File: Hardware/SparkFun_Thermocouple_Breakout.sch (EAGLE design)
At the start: 16 parts, among them U1 MAX31855K

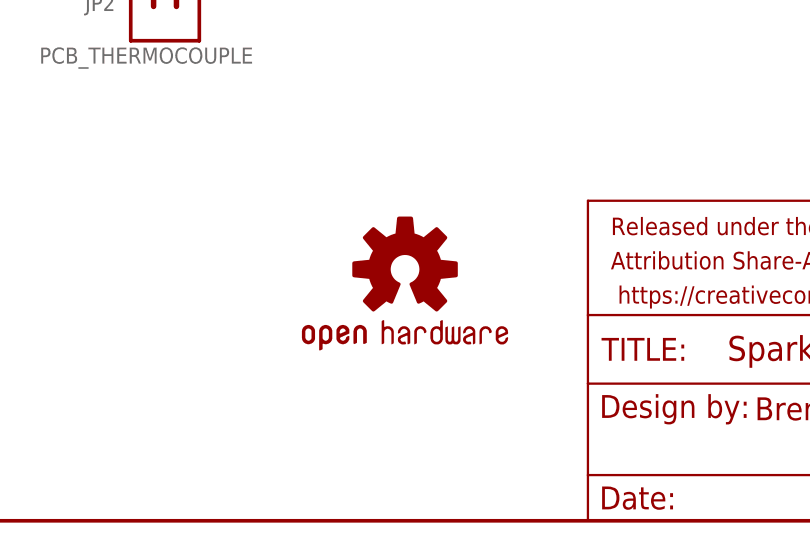
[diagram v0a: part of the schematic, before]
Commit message: Added more logos!
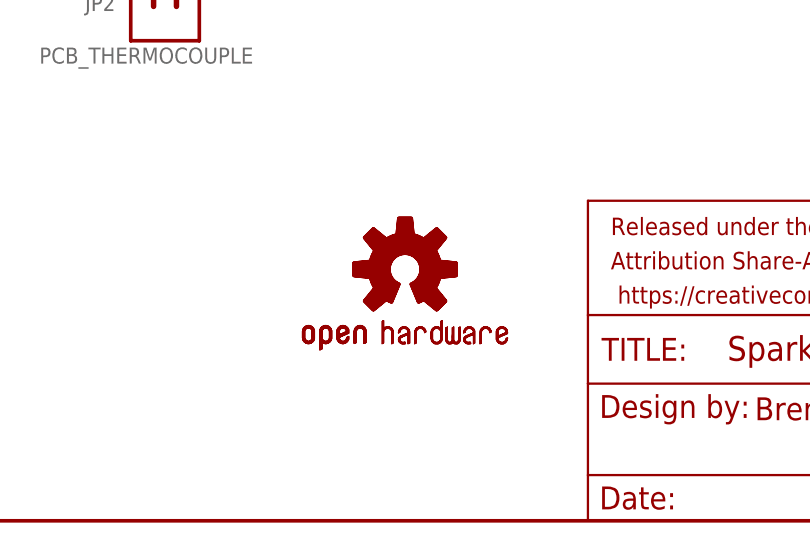
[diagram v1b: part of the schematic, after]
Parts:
- added LOGO4: OSHW-LOGOS, SparkFun-Aesthetics:OSHW-LOGOS
- U1: PROD_ID (none) -> IC-12578
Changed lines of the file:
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@@
 <part name="FID2" library="SparkFun-Aesthetics" deviceset="FIDUCIAL" device="1X2"/>
 <part name="C1" library="SparkFun-Capacitors" deviceset="0.1UF-25V(+80/-20%)(0603)" device="" value="0.1uF"/>
-<part name="U1" library="SparkFun-AnalogIC" deviceset="MAX31855K" device=""/>
+<part name="U1" library="SparkFun-AnalogIC" deviceset="MAX31855K" device="">
+<attribute name="PROD_ID" value="IC-12578"/>
+</part>
 <part name="GND2" library="SparkFun-Aesthetics" deviceset="GND" device=""/>
 <part name="JP1" library="SparkFun-Connectors" deviceset="M06" device="SILK_FEMALE_PTH" value="DNP"/>
@@
 <part name="JP2" library="Testing" deviceset="PCB_THERMOCOUPLE" device=""/>
 <part name="LOGO3" library="SparkFun-Aesthetics" deviceset="SFE_LOGO_NAME_FLAME" device=".1_INCH"/>
+<part name="LOGO4" library="SparkFun-Aesthetics" deviceset="OSHW-LOGO" device="S"/>
 </parts>
 <sheets>
@@
 <instance part="FID2" gate="G$1" x="241.3" y="25.4"/>
 <instance part="C1" gate="G$1" x="73.66" y="93.98" rot="MR0"/>
-<instance part="U1" gate="G$1" x="116.84" y="99.06"/>
+<instance part="U1" gate="G$1" x="116.84" y="99.06">
+<attribute name="PROD_ID" x="116.84" y="99.06" size="1.778" layer="96" display="off"/>
+</instance>
 <instance part="GND2" gate="1" x="73.66" y="86.36"/>
 <instance part="JP1" gate="G$1" x="162.56" y="96.52" rot="R180"/>
@@
 </instance>
 <instance part="LOGO3" gate="G$1" x="190.5" y="35.56"/>
+<instance part="LOGO4" gate="G$1" x="127" y="27.94"/>
 </instances>
 <busses>
